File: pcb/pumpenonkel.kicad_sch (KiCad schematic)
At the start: 21 parts, among them J1 Screw_Terminal_01x02, J10 NO_ON_JUMPER, J11 Screw_Terminal_01x02, J12 NO_ON_JUMPER, J13 Screw_Terminal_01x02, J14 Conn_01x02_Pin, J2 NO_ON_JUMPER, J3 Screw_Terminal_01x02, J4 NO_ON_JUMPER, J5 Screw_Terminal_01x02, J6 NO_ON_JUMPER, J7 Screw_Terminal_01x02, J8 NO_ON_JUMPER, J9 Screw_Terminal_01x02, K1 SANYOU_SRD_Form_C, K2 SANYOU_SRD_Form_C, K3 SANYOU_SRD_Form_C, K4 SANYOU_SRD_Form_C, K5 SANYOU_SRD_Form_C, K6 SANYOU_SRD_Form_C

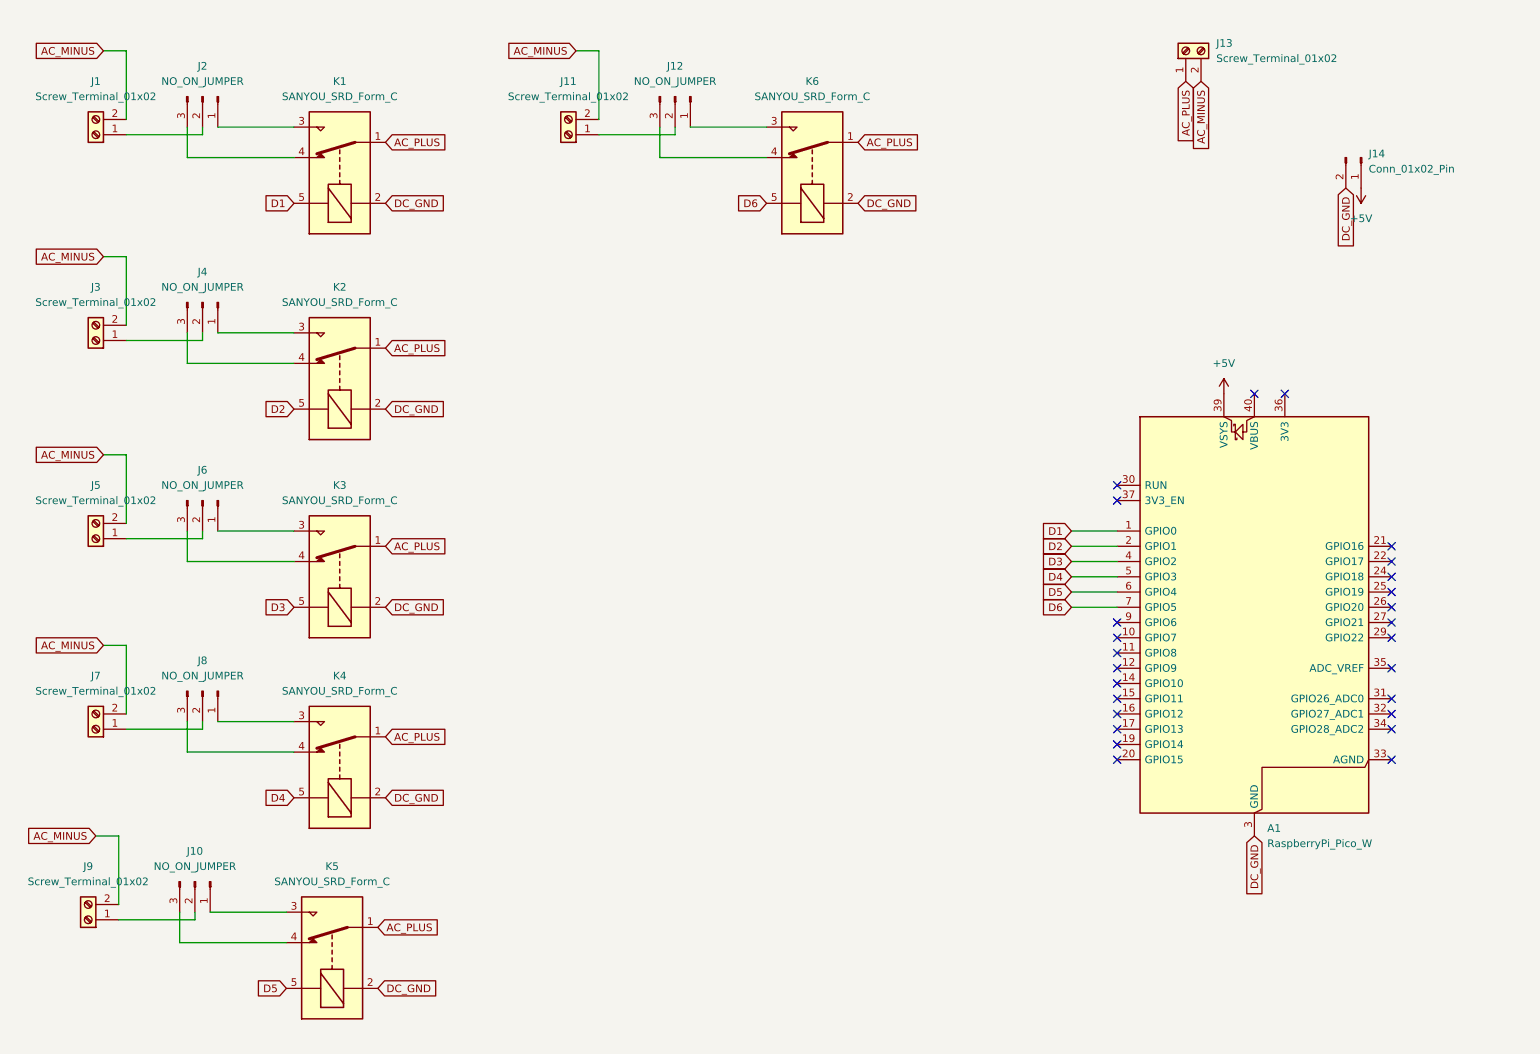
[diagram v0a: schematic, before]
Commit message: Update PCB
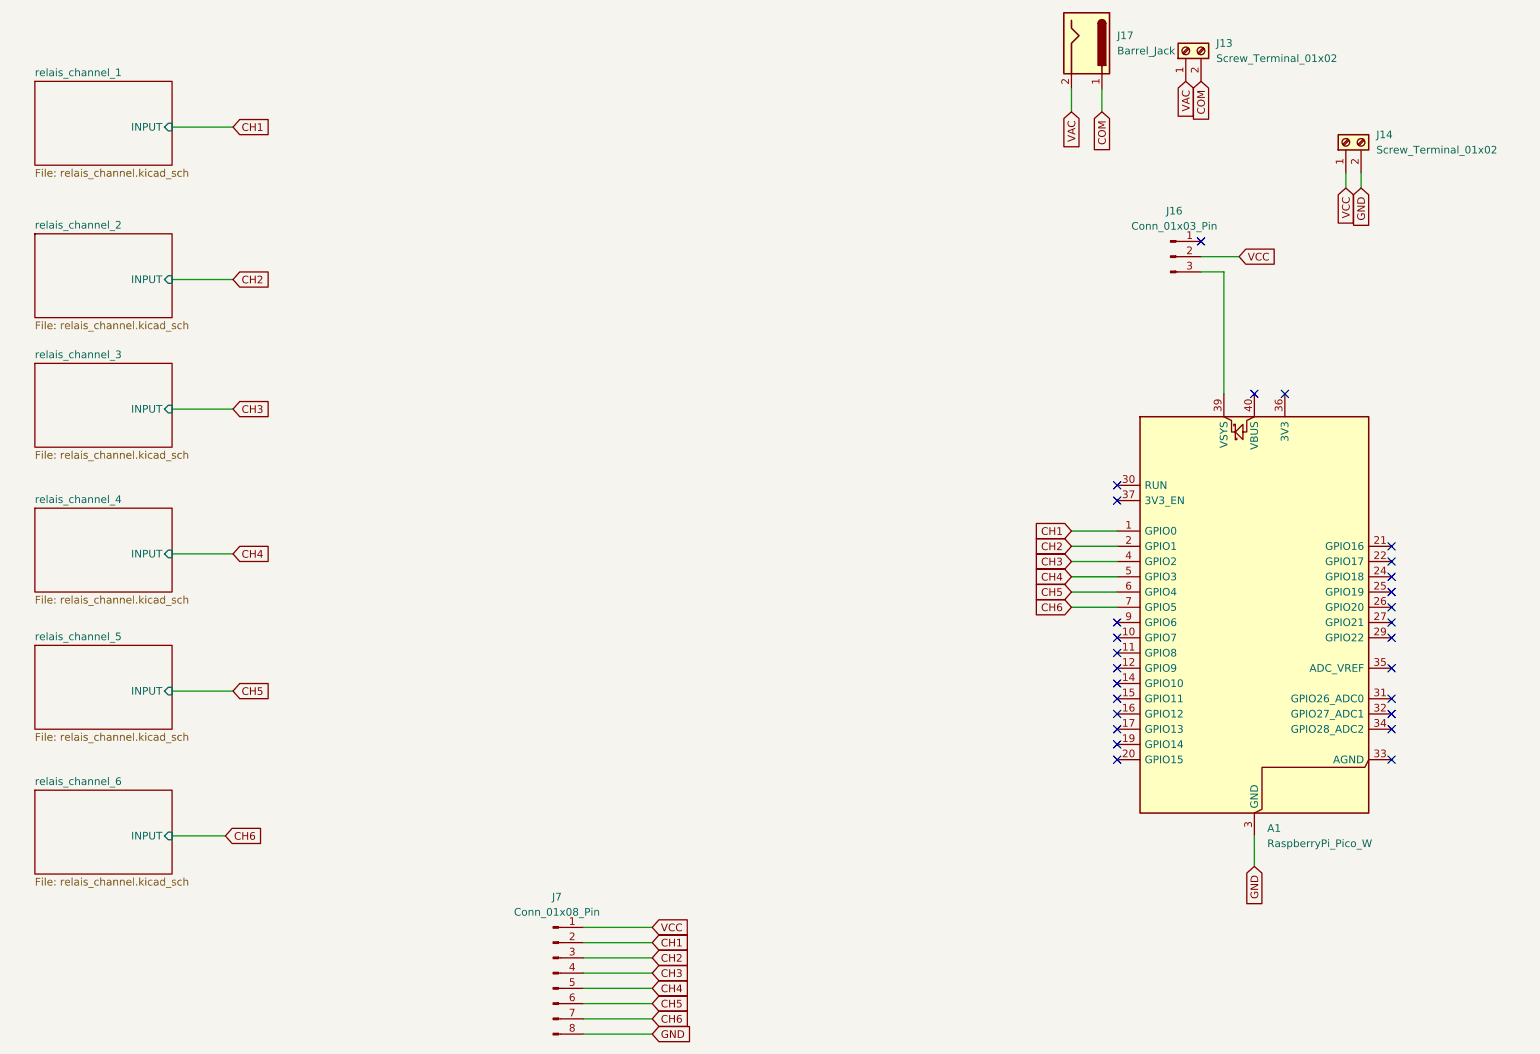
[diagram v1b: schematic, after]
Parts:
- removed J1, J11, J3, J5, J7, J9: Screw_Terminal_01x02, TerminalBlock:TerminalBlock_MaiXu_MX126-5.0-02P_1x02_P5.00mm, symbol Connector:Screw_Terminal_01x02
- removed J10, J12, J2, J4, J6, J8: NO_ON_JUMPER, Connector_PinHeader_2.54mm:PinHeader_1x03_P2.54mm_Horizontal, symbol Connector:Conn_01x03_Pin
- removed J14: Conn_01x02_Pin, TerminalBlock:TerminalBlock_MaiXu_MX126-5.0-02P_1x02_P5.00mm, symbol Connector:Conn_01x02_Pin
- removed K1, K2, K3, K4, K5, K6: SANYOU_SRD_Form_C, Relay_THT:Relay_SPDT_SANYOU_SRD_Series_Form_C, symbol Relay:SANYOU_SRD_Form_C
- added J14: Screw_Terminal_01x02, TerminalBlock:TerminalBlock_MaiXu_MX126-5.0-02P_1x02_P5.00mm, symbol Connector:Screw_Terminal_01x02
- added J16: Conn_01x03_Pin, Connector_PinHeader_2.54mm:PinHeader_1x03_P2.54mm_Vertical, symbol Connector:Conn_01x03_Pin
- added J17: Barrel_Jack, Connector_BarrelJack:BarrelJack_CUI_PJ-063AH_Horizontal, symbol Connector:Barrel_Jack
- added J7: Conn_01x08_Pin, Connector_PinHeader_2.54mm:PinHeader_1x08_P2.54mm_Vertical, symbol Connector:Conn_01x08_Pin
- A1: footprint Module:RaspberryPi_Pico_W_SMD_HandSolder -> Module:RaspberryPi_Pico_Common_THT
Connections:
- net +5V: no longer names the net of A1.39 (VSYS)
- net +5V: now also J16.3 (Pin_3)
- net AC_MINUS renamed COM
- net COM: now also J17.1
- net AC_PLUS renamed VAC
- net VAC: now also J17.2
- net D1 renamed CH1
- net CH1: now also J7.2 (Pin_2)
- net D2 renamed CH2
- net CH2: now also J7.3 (Pin_3)
- net D3 renamed CH3
- net CH3: now also J7.4 (Pin_4)
- net D4 renamed CH4
- net CH4: now also J7.5 (Pin_5)
- net D5 renamed CH5
- net CH5: now also J7.6 (Pin_6)
- net D6 renamed CH6
- net CH6: now also J7.7 (Pin_7)
- net DC_GND renamed GND
- net GND: now also J14.2 (Pin_2), J7.8 (Pin_8)
- new net VCC: J14.1 (Pin_1), J16.2 (Pin_2), J7.1 (Pin_1)
- no-connect marks 26 -> 27
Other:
- added sheet relais_channel_1 (relais_channel.kicad_sch)
- added sheet relais_channel_2 (relais_channel.kicad_sch)
- added sheet relais_channel_3 (relais_channel.kicad_sch)
- added sheet relais_channel_4 (relais_channel.kicad_sch)
- added sheet relais_channel_5 (relais_channel.kicad_sch)
- added sheet relais_channel_6 (relais_channel.kicad_sch)

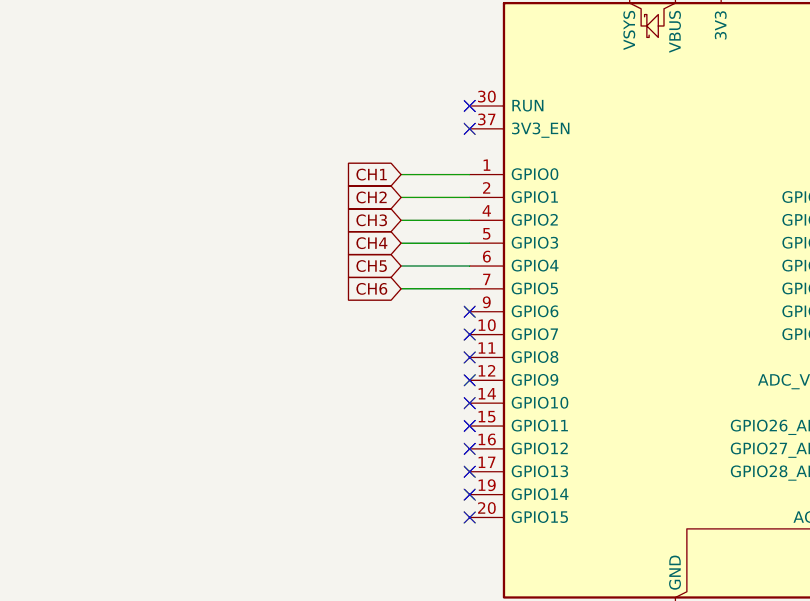
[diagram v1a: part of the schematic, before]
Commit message: Update pcb
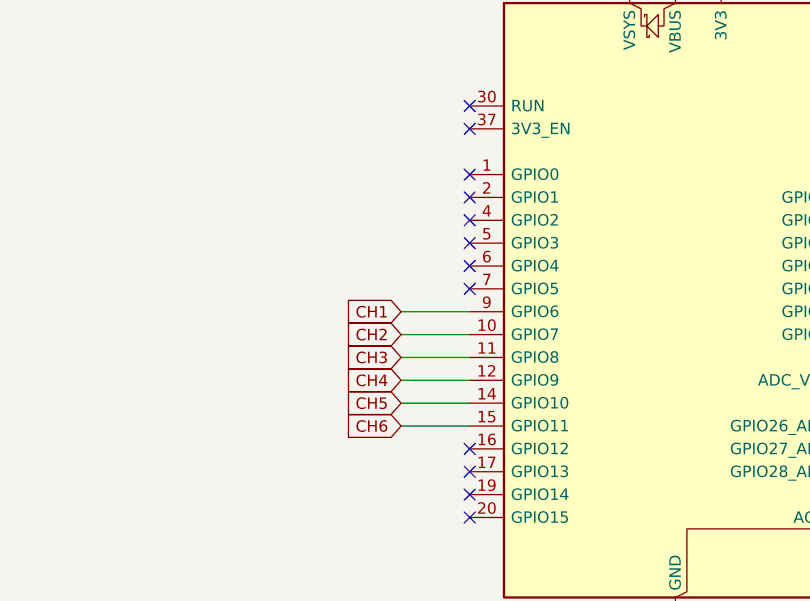
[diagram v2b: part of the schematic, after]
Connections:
- net CH1: now also A1.9 (GPIO6); no longer A1.1 (GPIO0)
- net CH2: now also A1.10 (GPIO7); no longer A1.2 (GPIO1)
- net CH3: now also A1.11 (GPIO8); no longer A1.4 (GPIO2)
- net CH4: now also A1.12 (GPIO9); no longer A1.5 (GPIO3)
- net CH5: now also A1.14 (GPIO10); no longer A1.6 (GPIO4)
- net CH6: now also A1.15 (GPIO11); no longer A1.7 (GPIO5)
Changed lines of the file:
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@@
 	(paper "A4")
 	(no_connect
-		(at 207.01 115.57)
-	)
-	(no_connect
 		(at 207.01 135.89)
 	)
@@
 	)
 	(no_connect
-		(at 207.01 123.19)
+		(at 207.01 105.41)
 	)
 	(no_connect
@@
 	)
 	(no_connect
-		(at 207.01 128.27)
+		(at 207.01 100.33)
 	)
 	(no_connect
@@
 	)
 	(no_connect
+		(at 207.01 102.87)
+	)
+	(no_connect
 		(at 207.01 133.35)
 	)
@@
 	)
 	(no_connect
-		(at 207.01 118.11)
-	)
-	(no_connect
 		(at 234.95 77.47)
 	)
 	(no_connect
-		(at 207.01 125.73)
-	)
-	(no_connect
 		(at 252.73 138.43)
 	)
@@
 	)
 	(no_connect
+		(at 207.01 107.95)
+	)
+	(no_connect
 		(at 229.87 77.47)
 	)
@@
 	)
 	(no_connect
-		(at 207.01 120.65)
+		(at 207.01 110.49)
+	)
+	(no_connect
+		(at 207.01 113.03)
 	)
 	(no_connect
@@
 	(wire
 		(pts
-			(xy 199.39 107.95) (xy 207.01 107.95)
-		)
-		(stroke
-			(width 0)
-			(type default)
-		)
-	)
-	(wire
-		(pts
 			(xy 49.53 33.02) (xy 59.69 33.02)
 		)
@@
 	(wire
 		(pts
+			(xy 199.39 123.19) (xy 207.01 123.19)
+		)
+		(stroke
+			(width 0)
+			(type default)
+		)
+	)
+	(wire
+		(pts
 			(xy 118.11 173.99) (xy 129.54 173.99)
 		)
@@
 	(wire
 		(pts
-			(xy 199.39 100.33) (xy 207.01 100.33)
-		)
-		(stroke
-			(width 0)
-			(type default)
-		)
-	)
-	(wire
-		(pts
 			(xy 220.98 54.61) (xy 227.33 54.61)
 		)
@@
 	(wire
 		(pts
+			(xy 199.39 128.27) (xy 207.01 128.27)
+		)
+		(stroke
+			(width 0)
+			(type default)
+		)
+	)
+	(wire
+		(pts
 			(xy 49.53 58.42) (xy 59.69 58.42)
 		)
@@
 	(wire
 		(pts
-			(xy 199.39 105.41) (xy 207.01 105.41)
-		)
-		(stroke
-			(width 0)
-			(type default)
-		)
-	)
-	(wire
-		(pts
 			(xy 118.11 184.15) (xy 129.54 184.15)
 		)
@@
 	(wire
 		(pts
+			(xy 199.39 118.11) (xy 207.01 118.11)
+		)
+		(stroke
+			(width 0)
+			(type default)
+		)
+	)
+	(wire
+		(pts
+			(xy 199.39 115.57) (xy 207.01 115.57)
+		)
+		(stroke
+			(width 0)
+			(type default)
+		)
+	)
+	(wire
+		(pts
 			(xy 204.47 26.67) (xy 204.47 30.48)
 		)
@@
 	(wire
 		(pts
-			(xy 199.39 110.49) (xy 207.01 110.49)
+			(xy 199.39 125.73) (xy 207.01 125.73)
 		)
 		(stroke
@@
 	(wire
 		(pts
-			(xy 199.39 102.87) (xy 207.01 102.87)
+			(xy 199.39 120.65) (xy 207.01 120.65)
 		)
 		(stroke
@@
 	(wire
 		(pts
-			(xy 199.39 113.03) (xy 207.01 113.03)
-		)
-		(stroke
-			(width 0)
-			(type default)
-		)
-	)
-	(wire
-		(pts
 			(xy 199.39 26.67) (xy 199.39 30.48)
 		)
@@
 	(global_label "CH4"
 		(shape input)
-		(at 199.39 107.95 180)
-		(fields_autoplaced yes)
-		(effects
-			(font
-				(size 1.27 1.27)
-			)
-			(justify right)
-		)
-		(property "Intersheetrefs" "${INTERSHEET_REFS}"
-			(at 192.5948 107.95 0)
+		(at 199.39 123.19 180)
+		(fields_autoplaced yes)
+		(effects
+			(font
+				(size 1.27 1.27)
+			)
+			(justify right)
+		)
+		(property "Intersheetrefs" "${INTERSHEET_REFS}"
+			(at 192.5948 123.19 0)
 			(effects
 				(font
@@
 	(global_label "CH2"
 		(shape input)
-		(at 199.39 102.87 180)
-		(fields_autoplaced yes)
-		(effects
-			(font
-				(size 1.27 1.27)
-			)
-			(justify right)
-		)
-		(property "Intersheetrefs" "${INTERSHEET_REFS}"
-			(at 192.5948 102.87 0)
+		(at 199.39 118.11 180)
+		(fields_autoplaced yes)
+		(effects
+			(font
+				(size 1.27 1.27)
+			)
+			(justify right)
+		)
+		(property "Intersheetrefs" "${INTERSHEET_REFS}"
+			(at 192.5948 118.11 0)
 			(effects
 				(font
@@
 	(global_label "CH6"
 		(shape input)
-		(at 199.39 113.03 180)
-		(fields_autoplaced yes)
-		(effects
-			(font
-				(size 1.27 1.27)
-			)
-			(justify right)
-		)
-		(property "Intersheetrefs" "${INTERSHEET_REFS}"
-			(at 192.5948 113.03 0)
+		(at 199.39 128.27 180)
+		(fields_autoplaced yes)
+		(effects
+			(font
+				(size 1.27 1.27)
+			)
+			(justify right)
+		)
+		(property "Intersheetrefs" "${INTERSHEET_REFS}"
+			(at 192.5948 128.27 0)
 			(effects
 				(font
@@
 	(global_label "CH5"
 		(shape input)
-		(at 199.39 110.49 180)
-		(fields_autoplaced yes)
-		(effects
-			(font
-				(size 1.27 1.27)
-			)
-			(justify right)
-		)
-		(property "Intersheetrefs" "${INTERSHEET_REFS}"
-			(at 192.5948 110.49 0)
+		(at 199.39 125.73 180)
+		(fields_autoplaced yes)
+		(effects
+			(font
+				(size 1.27 1.27)
+			)
+			(justify right)
+		)
+		(property "Intersheetrefs" "${INTERSHEET_REFS}"
+			(at 192.5948 125.73 0)
 			(effects
 				(font
@@
 	(global_label "CH3"
 		(shape input)
-		(at 199.39 105.41 180)
-		(fields_autoplaced yes)
-		(effects
-			(font
-				(size 1.27 1.27)
-			)
-			(justify right)
-		)
-		(property "Intersheetrefs" "${INTERSHEET_REFS}"
-			(at 192.5948 105.41 0)
+		(at 199.39 120.65 180)
+		(fields_autoplaced yes)
+		(effects
+			(font
+				(size 1.27 1.27)
+			)
+			(justify right)
+		)
+		(property "Intersheetrefs" "${INTERSHEET_REFS}"
+			(at 192.5948 120.65 0)
 			(effects
 				(font
@@
 	(global_label "CH1"
 		(shape input)
-		(at 199.39 100.33 180)
-		(fields_autoplaced yes)
-		(effects
-			(font
-				(size 1.27 1.27)
-			)
-			(justify right)
-		)
-		(property "Intersheetrefs" "${INTERSHEET_REFS}"
-			(at 192.5948 100.33 0)
-			(effects
-				(font
+		(at 199.39 115.57 180)
+		(fields_autoplaced yes)
+		(effects
+			(font
+				(size 1.27 1.27)
+			)
+			(justify right)
+		)
+		(property "Intersheetrefs" "${INTERSHEET_REFS}"
+			(at 192.5948 115.57 0)
+			(effects
+				(font
